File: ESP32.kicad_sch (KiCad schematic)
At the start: 5 parts, among them U1 ESP32-C6-MINI-1/U

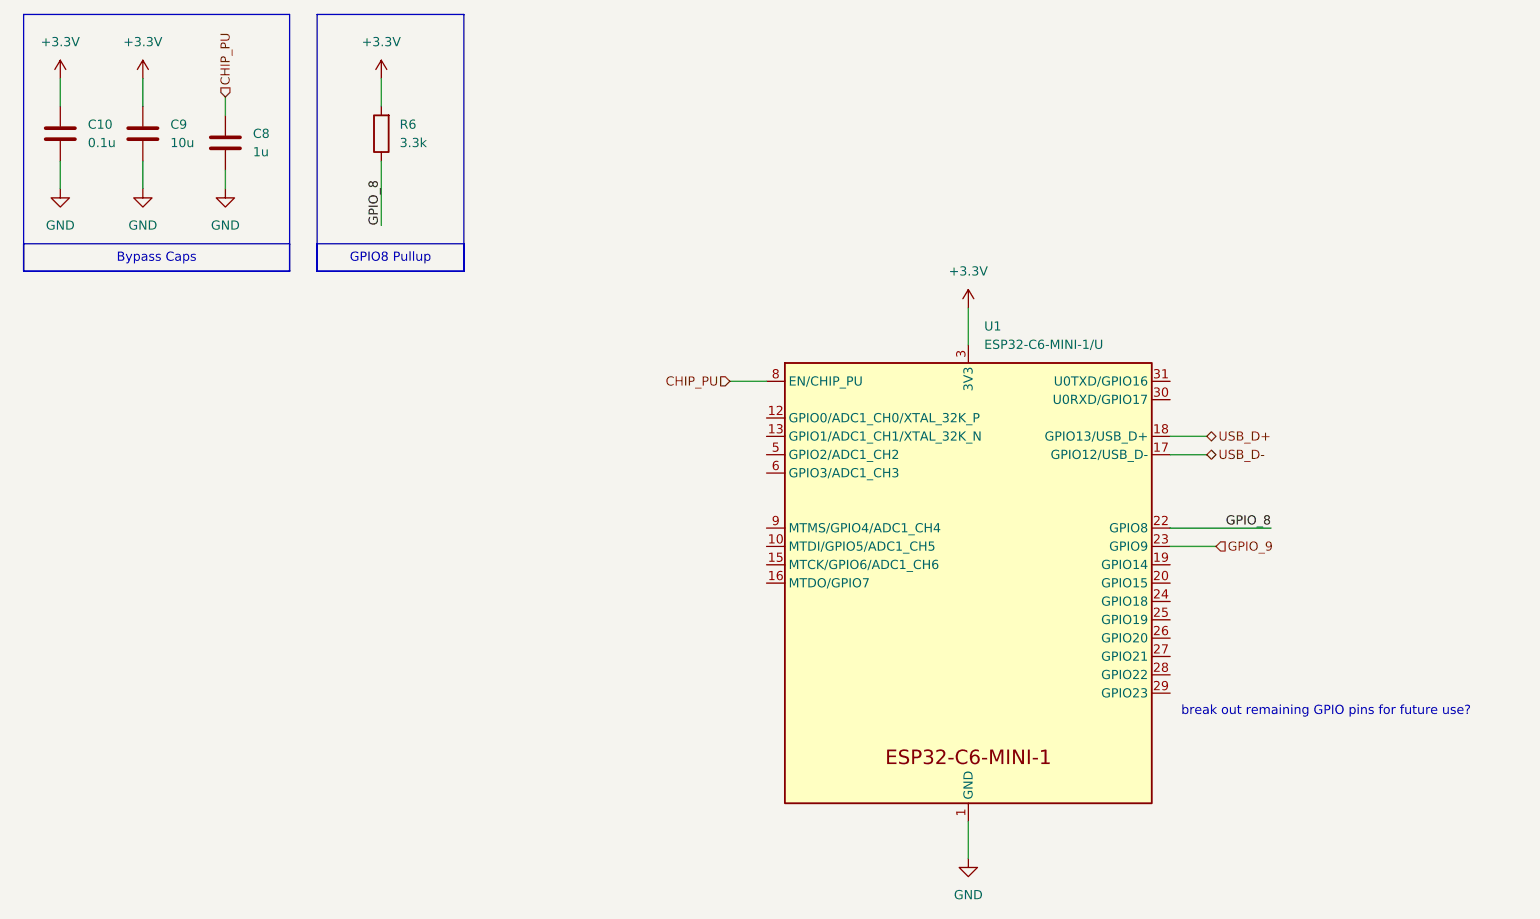
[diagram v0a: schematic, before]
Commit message: finished sch? (need P/Ns)
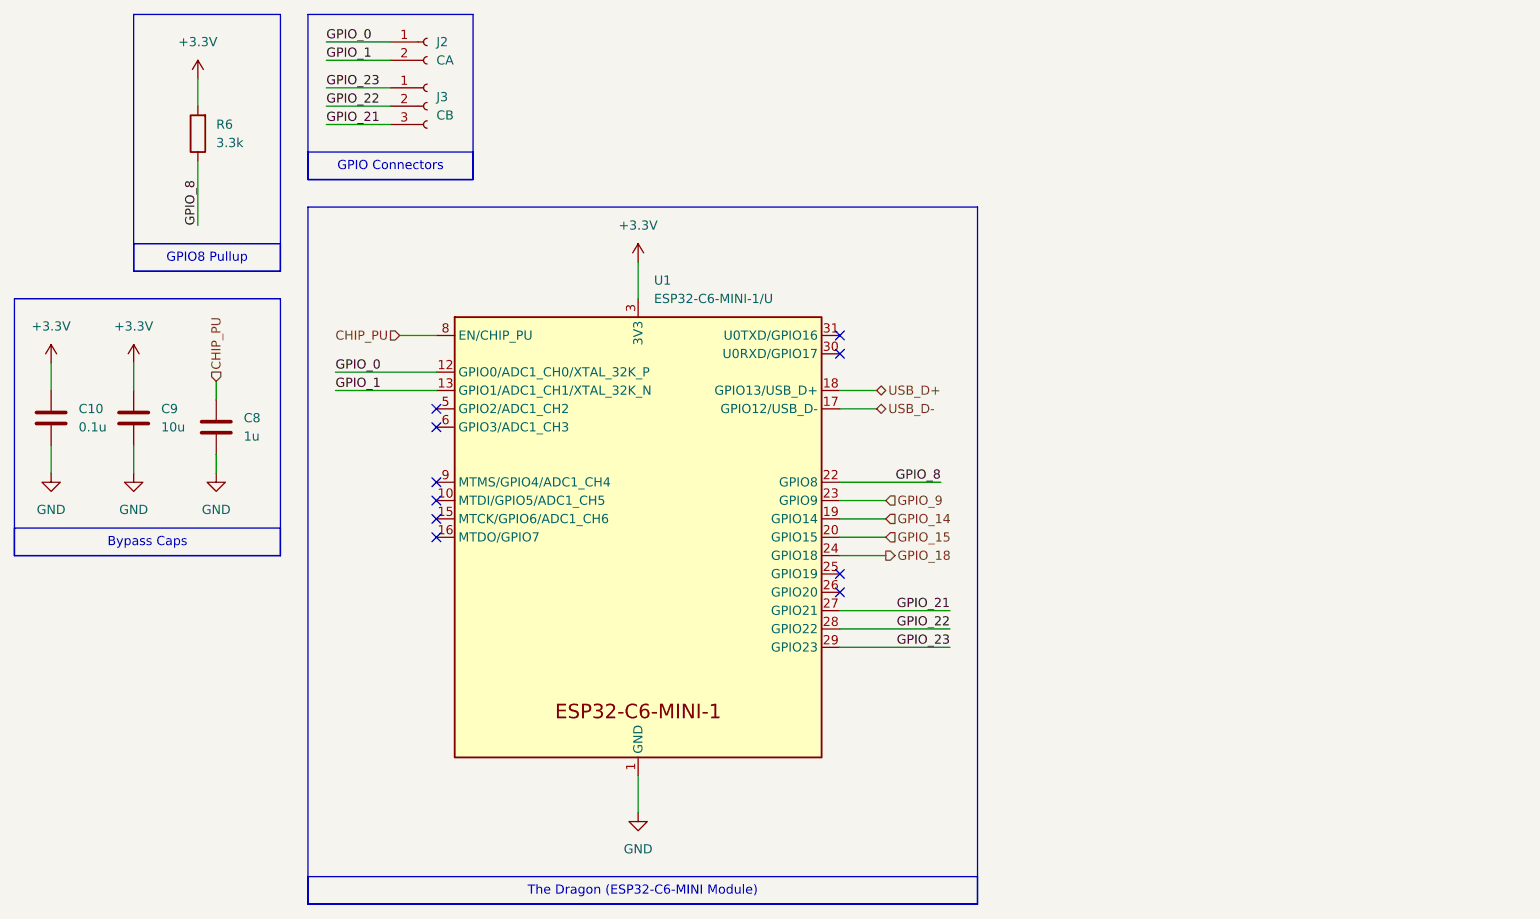
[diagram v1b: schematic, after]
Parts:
- added J2: CA, symbol Connector:Conn_01x02_Socket
- added J3: CB, symbol Connector:Conn_01x03_Socket
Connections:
- net GPIO_0: now reaches U1.12 (GPIO0/ADC1_CH0/XTAL_32K_P)
- net GPIO_0: now also J2.1 (Pin_1)
- net GPIO_1: now reaches U1.13 (GPIO1/ADC1_CH1/XTAL_32K_N)
- net GPIO_1: now also J2.2 (Pin_2)
- net GPIO_14: now reaches U1.19 (GPIO14)
- net GPIO_15: now reaches U1.20 (GPIO15)
- net GPIO_18: now reaches U1.24 (GPIO18)
- net GPIO_21: now reaches U1.27 (GPIO21)
- net GPIO_21: now also J3.3 (Pin_3)
- net GPIO_22: now reaches U1.28 (GPIO22)
- net GPIO_22: now also J3.2 (Pin_2)
- net GPIO_23: now reaches U1.29 (GPIO23)
- net GPIO_23: now also J3.1 (Pin_1)
- no-connect marks 0 -> 10
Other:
- note removed: "break out remaining GPIO pins for future use?"
- moved on the sheet: C10, C8, C9, R6, U1
